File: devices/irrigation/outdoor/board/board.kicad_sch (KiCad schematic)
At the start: 12 parts, among them J1 Cap Sensor, J10 Relay Board, J11 Cap Sensor, J2 Cap Sensor, J3 Cap Sensor, J4 GME12864, J5 BUCK Conv, J6 Relay Board, J7 Relay Board, J8 Relay Board, J9 Barrel_Jack_MountingPin, U1 ESP32-C3-DevKitM-1

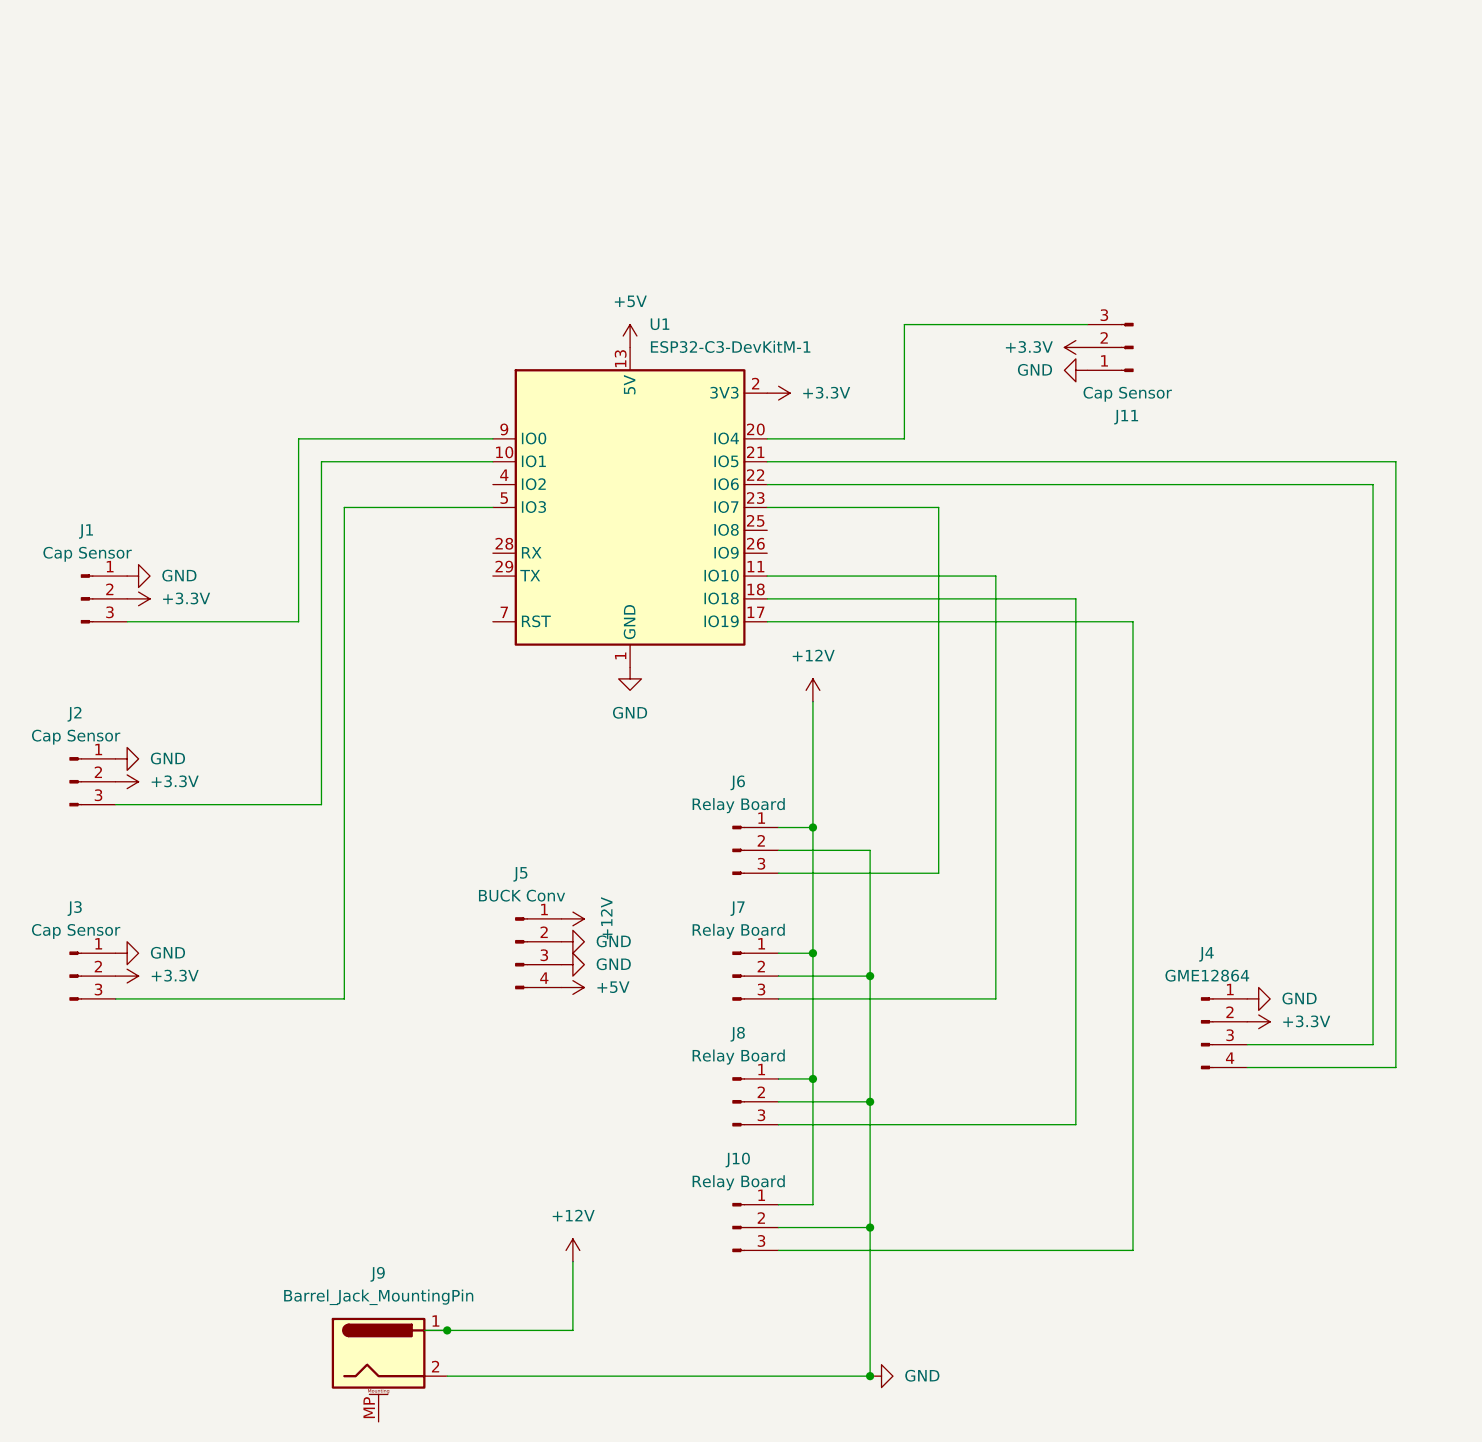
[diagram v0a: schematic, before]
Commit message: wasdf
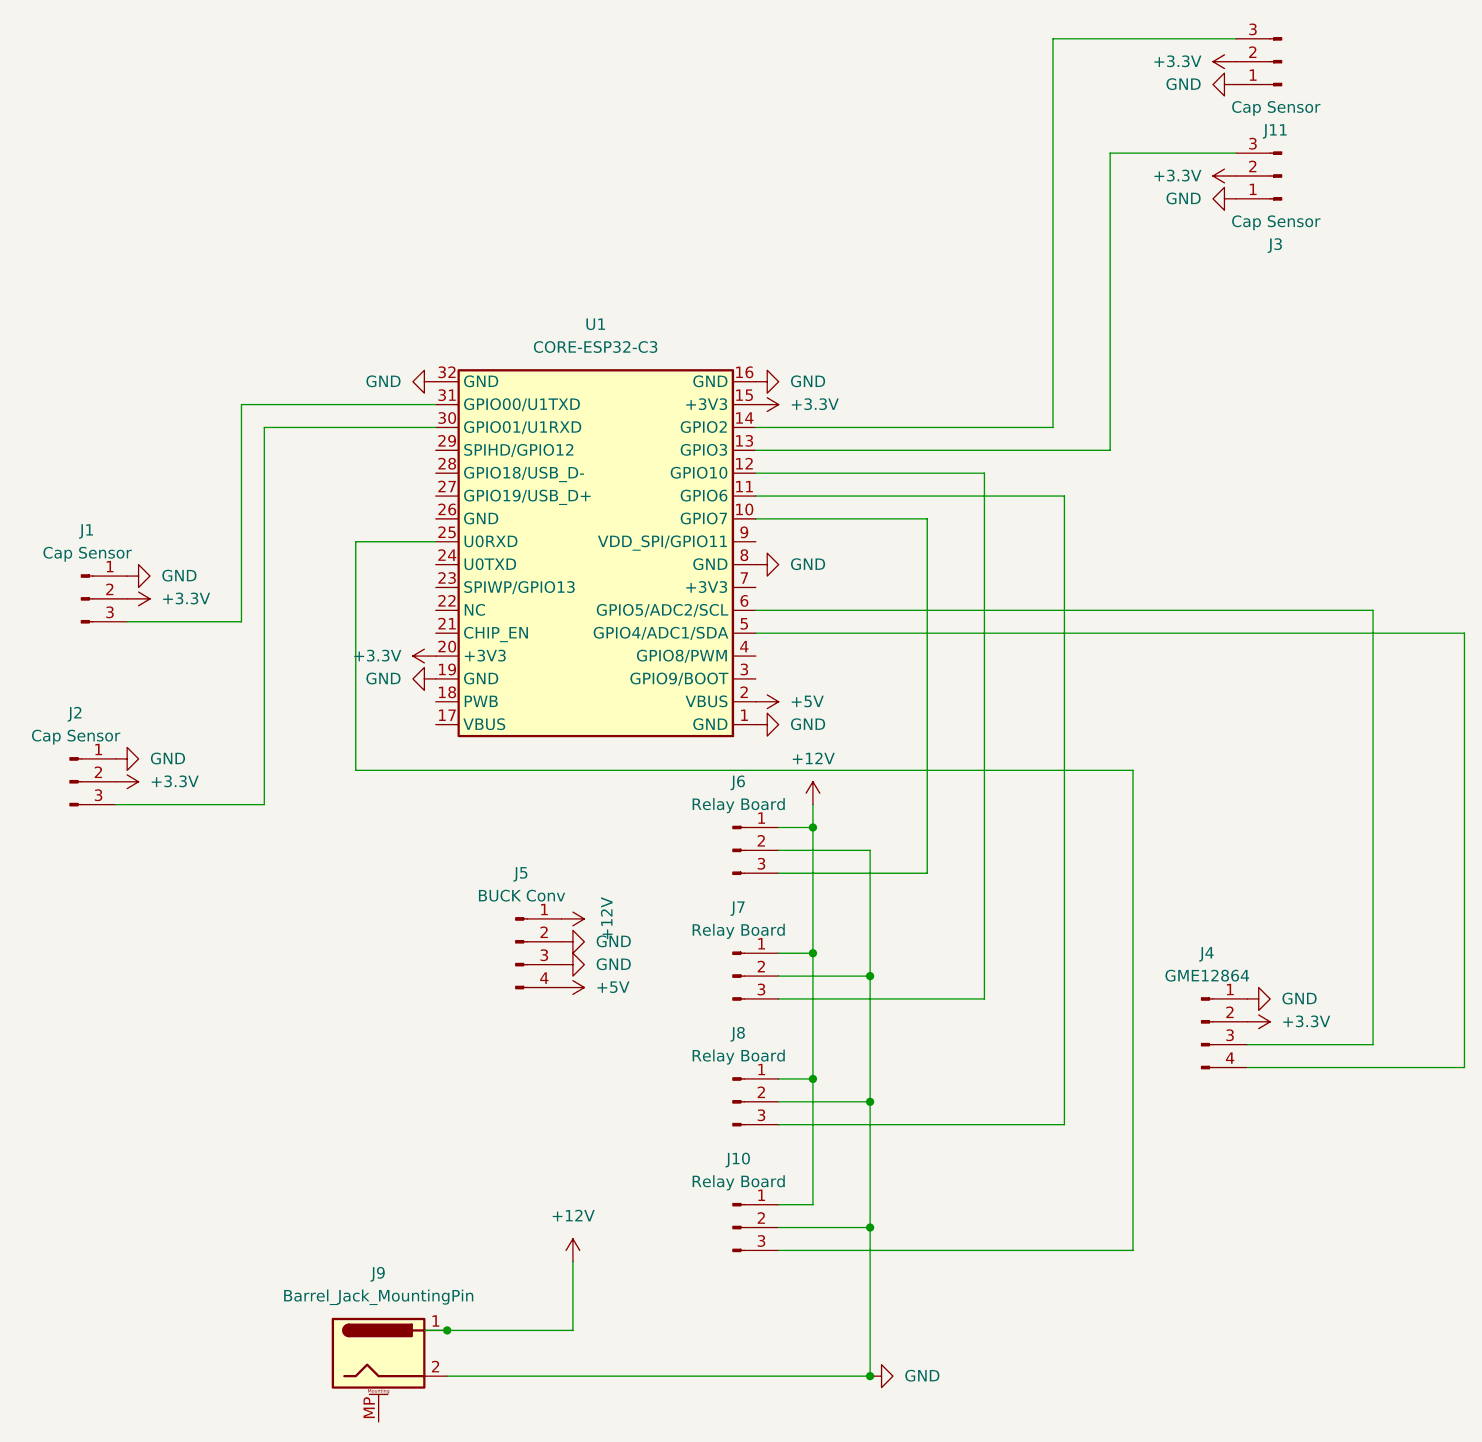
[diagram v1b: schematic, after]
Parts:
- removed U1: ESP32-C3-DevKitM-1, RF_Module:ESP32-C3-DevKitM-1, symbol RF_Module:ESP32-C3-DevKitM-1
- added U1: CORE-ESP32-C3, CORE-ESP32-C3:CORE-ESP32-C3, symbol CORE-ESP32-C3:CORE-ESP32-C3
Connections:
- net +3.3V: now also U1.15 (+3V3), U1.20 (+3V3)
- net +5V: now also U1.2 (VBUS)
- net GND: now also U1.1 (GND), U1.16 (GND), U1.19 (GND), U1.32 (GND), U1.8 (GND)
- net at J2.3 (Pin_3): now also U1.30 (GPIO01/U1RXD)
- net at J7.3 (Pin_3): now also U1.12 (GPIO10)
- net at J10.3 (Pin_3): now also U1.25 (U0RXD)
- net at J8.3 (Pin_3): now also U1.11 (GPIO6)
- net at J11.3 (Pin_3): now also U1.14 (GPIO2)
- net at J4.4 (Pin_4): now also U1.5 (GPIO4/ADC1/SDA)
- net at J4.3 (Pin_3): now also U1.6 (GPIO5/ADC2/SCL)
- net at J6.3 (Pin_3): now also U1.10 (GPIO7)
- net at J3.3 (Pin_3): now also U1.13 (GPIO3)
- net at J1.3 (Pin_3): now also U1.31 (GPIO00/U1TXD)
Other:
- moved on the sheet: J11, J3
